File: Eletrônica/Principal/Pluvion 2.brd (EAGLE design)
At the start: 63.5 x 72.1 mm, 15 parts, among them Q1 PFET, Q2 NFET

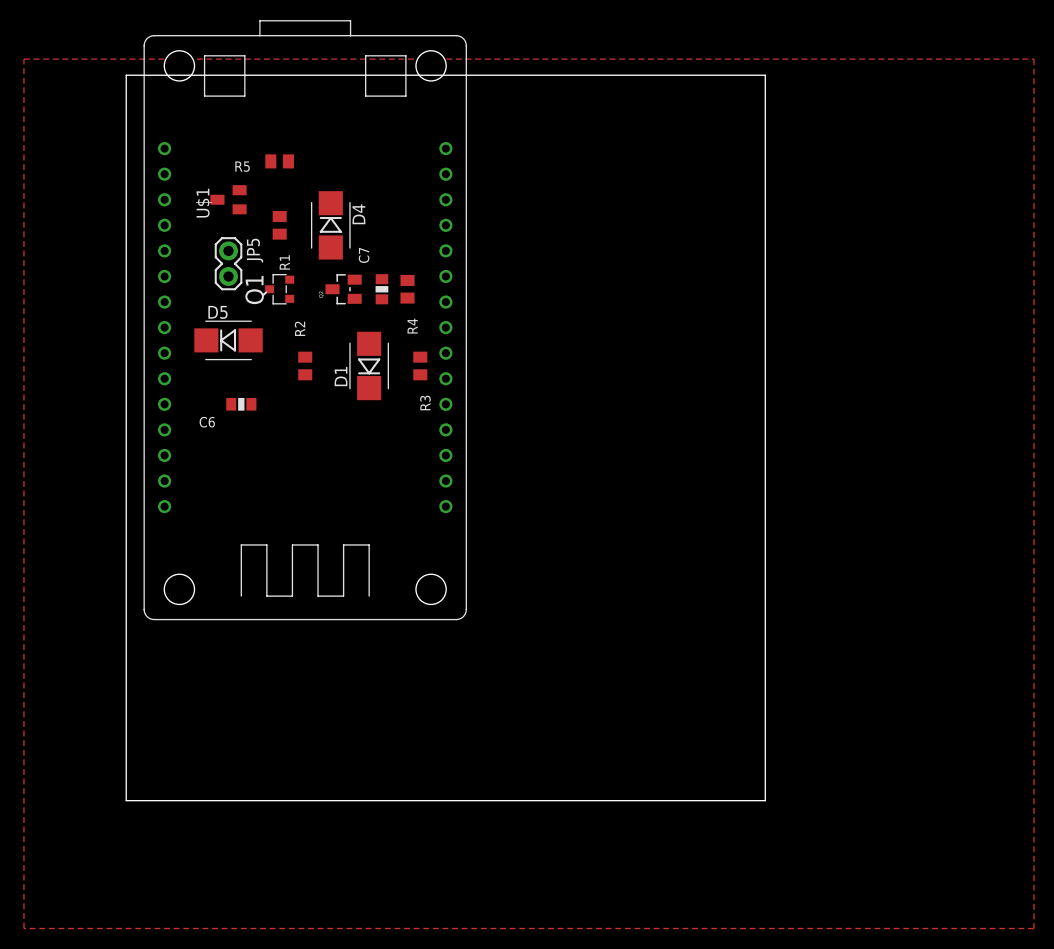
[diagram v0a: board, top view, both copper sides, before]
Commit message: Pluvion V2
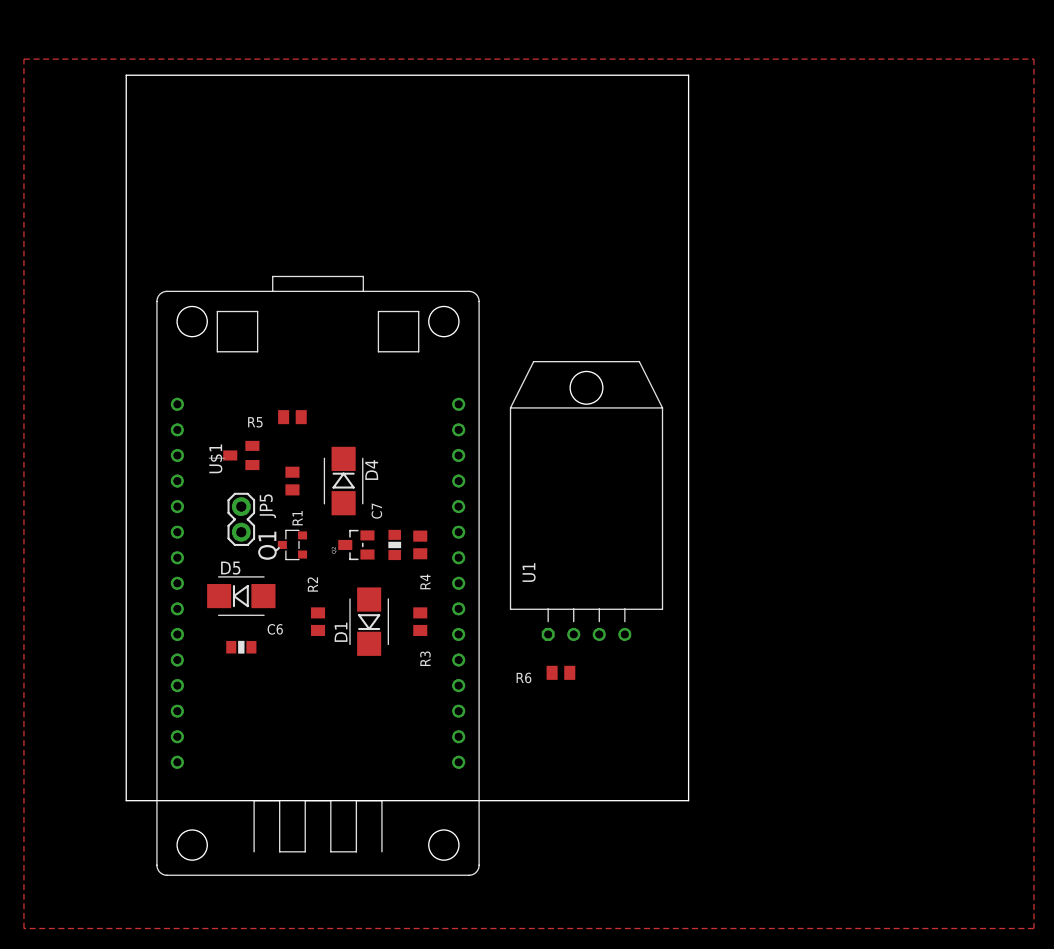
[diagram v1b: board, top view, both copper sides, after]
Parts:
- added R6: (no value), wes:R0805
- added U1: (no value), RHT03_DHT-22_AM2302:RHT03_DHT-22/RA
- moved U$2 25.4 mm to (19.1, 21.6)
- moved C7 25.4 mm to (26.7, 25.4)
- moved D4 25.4 mm to (21.6, 31.8)
- moved D5 25.4 mm to (11.4, 20.3)
- moved JP5 25.4 mm to (11.4, 29.2)
- moved Q1 25.4 mm to (16.5, 25.4)
- moved Q2 25.4 mm to (22.9, 25.4)
- moved R1 25.4 mm to (16.5, 31.8)
- moved R2 25.4 mm to (19.1, 17.8)
- moved R4 25.4 mm to (29.2, 25.4)
- moved R5 25.4 mm to (16.5, 38.1)
- moved U$1 25.4 mm to (11.4, 34.3)
- moved D1 25.4 mm to (24.1, 17.8)
- moved R3 25.4 mm to (29.2, 17.8)
- moved C6 24.1 mm to (11.4, 15.2), turned to 0 degrees
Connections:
- new net N$17: R6.1, U1.DATA
- net +3V3: now also R6.2, U1.VDD
- net GND: now also U1.GND
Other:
- board size 63.5 x 72.1 mm -> 55.9 x 72.1 mm

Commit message: Pluvion V2 ready for prototyping
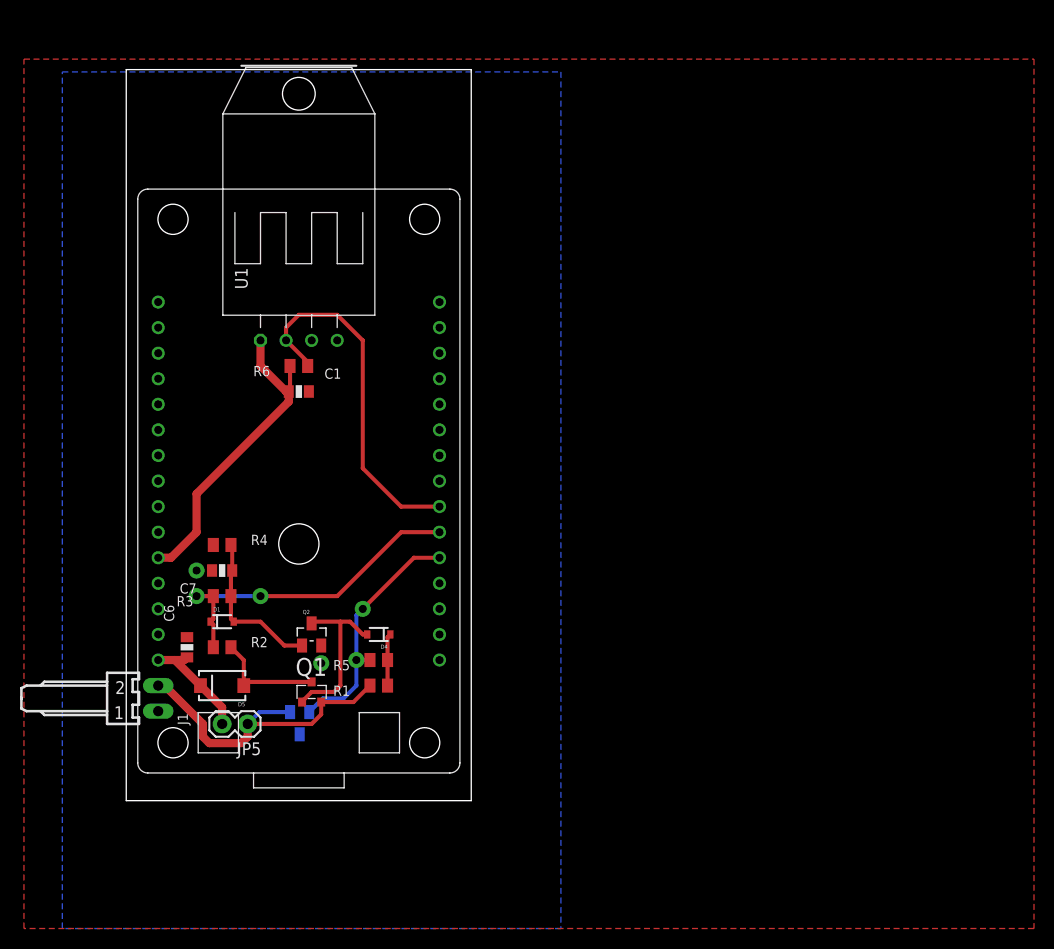
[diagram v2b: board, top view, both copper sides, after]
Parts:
- added C1: 10uF 10V, wes:C0805
- added J1: 22-05-7028-02, con-molex:7395-02
- D1, D4: device SparkFun-DiscreteSemi:SMB-DIODE -> SparkFun-DiscreteSemi:SOD-323
- D5: device SparkFun-DiscreteSemi:SMB-DIODE -> SparkFun-DiscreteSemi:SMA-DIODE
- moved U1 40.9 mm to (17.1, 45.7)
- moved R6 40.1 mm to (17.1, 43.2)
- moved U$1 27.2 mm to (17.2, 7.70), flipped to the bottom, turned to 180 degrees
- moved R5 25.6 mm to (25.1, 14.0)
- moved R1 22.1 mm to (25.1, 11.4), turned to 180 degrees
- moved JP5 21.6 mm to (12.1, 7.62), turned to 180 degrees
- moved R3 19.8 mm to (9.53, 20.3), turned to 180 degrees
- moved R4 19.7 mm to (9.53, 25.4), turned to 0 degrees
- moved C7 17.3 mm to (9.53, 22.9), turned to 180 degrees
- moved D4 15.6 mm to (25.1, 16.5), turned to 180 degrees
- moved Q1 14.7 mm to (18.4, 10.8), turned to 0 degrees
- moved D1 14.6 mm to (9.53, 17.8), turned to 0 degrees
- moved U$2 10.3 mm to (17.1, 31.8), turned to 180 degrees
- moved Q2 9.94 mm to (18.4, 16.5), turned to 0 degrees
- moved R2 9.86 mm to (9.53, 15.2), turned to 0 degrees
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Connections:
- removed net N$14 (its old number): U$2.D8
- removed net N$17 (its old number): R6.1, U1.DATA
- removed net N$18: U$2.3V@3
- removed net N$33: U$2.VIN
- new net +5V: C6.1, D5.C, JP5.2, U$2.VIN
- new net DHT_DATA: R6.1, U$2.D6, U1.DATA
- net +3V3: now also C1.1, U$2.3V@3; no longer C6.1, D5.C, JP5.2
- net ARD_OFF: now also D1.1, U$2.D7; no longer D1.C
- net BUTTONS: now also D4.2; no longer D4.A
- net GND: now also C1.2, J1.1; no longer U$2.G@3, U$2.G@4
- net HALL: now also U$2.D8
- net N$12: now also U$2.G@3; no longer U$2.D6
- net N$13: now also U$2.G@4; no longer U$2.D7
- net N$2: now also D1.2; no longer D1.A
- net N$8: now also D4.1; no longer D4.C
- net VIN: now also J1.2
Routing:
- net DHT_DATA: track 0.00 -> 35.8 mm
- net ARD_OFF: track 0.00 -> 33.7 mm, vias 0 -> 2
- net VIN: track 0.00 -> 32.7 mm
- net +3V3: track 0.00 -> 31.6 mm
- net HALL: track 0.00 -> 24.7 mm, vias 0 -> 2
- net BUTTONS: track 0.00 -> 17.0 mm
- net N$2: track 0.00 -> 15.6 mm
- net +5V: track 0.00 -> 11.3 mm
- net N$1: track 0.00 -> 11.2 mm
- net N$8: track 0.00 -> 5.19 mm
- added copper zone on layer 16, net GND
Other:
- board size 55.9 x 72.1 mm -> 34.3 x 72.6 mm
